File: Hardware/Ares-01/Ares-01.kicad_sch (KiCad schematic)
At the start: 25 parts, among them J1 BTS7960_1, J12 XT60, J13 TCRT5000_1, J14 TCRT5000_2, J15 TCRT5000_3, J2 BTS7960_2, J3 Sharp, J4 Sharp, J5 Sharp, J6 Sharp, J7 Sharp, J8 Qtr8a, J9 Ssd1306 Arduino Pic, SW1 Switch, SW2 SW_Push, SW3 SW_Push, U1 L7805, U3 CD74HC4067M

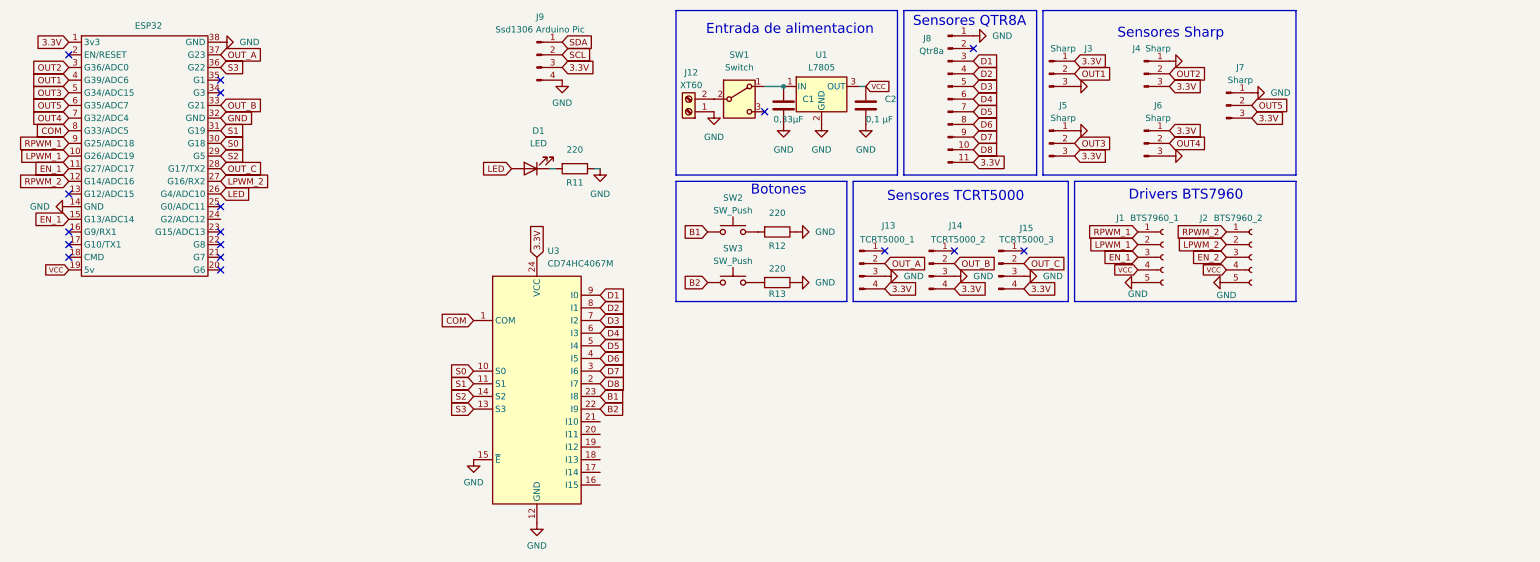
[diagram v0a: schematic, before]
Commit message: primer version del pcb
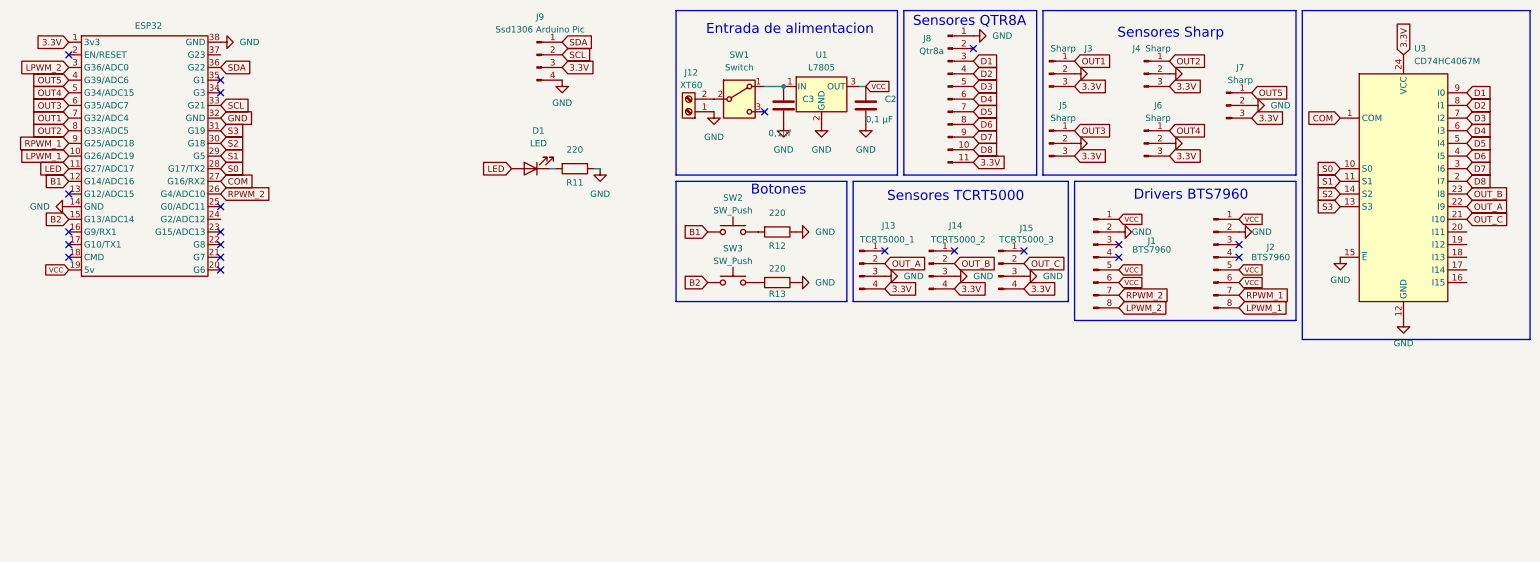
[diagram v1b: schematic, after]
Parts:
- removed C1: 0,33µF, symbol Device:C
- removed J1: BTS7960_1, Connector_IDC:IDC-Header_2x04_P2.54mm_Vertical, symbol Connector:Conn_01x05_Socket
- removed J2: BTS7960_2, Connector_IDC:IDC-Header_2x04_P2.54mm_Vertical, symbol Connector:Conn_01x05_Socket
- added C3: 0,1uf, Capacitor_SMD:C_1206_3216Metric_Pad1.33x1.80mm_HandSolder, symbol Device:C
- added J1, J2: BTS7960, Connector_IDC:IDC-Header_2x04_P2.54mm_Vertical, symbol Connector:Conn_01x08_Pin
- C2: footprint (none) -> Capacitor_SMD:C_1206_3216Metric_Pad1.33x1.80mm_HandSolder
- D1: footprint Connector_JST:JST_EH_S2B-EH_1x02_P2.50mm_Horizontal -> Connector_JST:JST_EH_B2B-EH-A_1x02_P2.50mm_Vertical
- J13, J14, J15: footprint Connector_JST:JST_EH_S4B-EH_1x04_P2.50mm_Horizontal -> Connector_JST:JST_EH_B4B-EH-A_1x04_P2.50mm_Vertical
- J3, J4, J5, J6, J7: footprint Connector_JST:JST_EH_S3B-EH_1x03_P2.50mm_Horizontal -> Connector_JST:JST_EH_B3B-EH-A_1x03_P2.50mm_Vertical
- J8: footprint Connector_JST:JST_EH_S11B-EH_1x11_P2.50mm_Horizontal -> Connector_JST:JST_EH_B10B-EH-A_1x10_P2.50mm_Vertical
- SW1: footprint EESTN5 2:SW_SPDT_TH_Vertical -> EESTN5:SW_SPDT_TH_Vertical
- SW2, SW3: footprint EESTN5 2:PUSH_SWITCH_THT -> EESTN5:PUSH_SWITCH_THT
- U3: footprint Package_SO:SOIC-24W_7.5x15.4mm_P1.27mm -> RamLib:CD74HC4067_module
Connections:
- net 3.3V: now also J3.3 (Pin_3), J6.3 (Pin_3); no longer J3.1 (Pin_1), J6.1 (Pin_1)
- net B1: now also ESP32.12 (G14/ADC16); no longer U3.23 (I8)
- net B2: now also ESP32.15 (G13/ADC14); no longer U3.22 (I9)
- net COM: now also ESP32.27 (G16/RX2); no longer ESP32.8 (G33/ADC5)
- net GND: now also J3.2 (Pin_2), J4.2 (Pin_2), J5.2 (Pin_2), J6.2 (Pin_2), J7.2 (Pin_2), C3.2, J1.2 (Pin_2), J2.2 (Pin_2); no longer J3.3 (Pin_3), J4.1 (Pin_1), J5.1 (Pin_1), J6.3 (Pin_3), J7.1 (Pin_1)
- net LED: now also ESP32.11 (G27/ADC17); no longer ESP32.26 (G4/ADC10)
- net LPWM_1: now also J2.8 (Pin_8)
- net LPWM_2: now also ESP32.3 (G36/ADC0), J1.8 (Pin_8); no longer ESP32.27 (G16/RX2)
- net OUT1: now also ESP32.7 (G32/ADC4), J3.1 (Pin_1); no longer ESP32.4 (G39/ADC6), J3.2 (Pin_2)
- net OUT2: now also ESP32.8 (G33/ADC5), J4.1 (Pin_1); no longer ESP32.3 (G36/ADC0), J4.2 (Pin_2)
- net OUT3: now also ESP32.6 (G35/ADC7), J5.1 (Pin_1); no longer ESP32.5 (G34/ADC15), J5.2 (Pin_2)
- net OUT4: now also ESP32.5 (G34/ADC15), J6.1 (Pin_1); no longer ESP32.7 (G32/ADC4), J6.2 (Pin_2)
- net OUT5: now also ESP32.4 (G39/ADC6), J7.1 (Pin_1); no longer ESP32.6 (G35/ADC7), J7.2 (Pin_2)
- net OUT_A: now also U3.22 (I9); no longer ESP32.37 (G23)
- net OUT_B: now also U3.23 (I8); no longer ESP32.33 (G21)
- net OUT_C: now also U3.21 (I10); no longer ESP32.28 (G17/TX2)
- net RPWM_1: now also J2.7 (Pin_7)
- net RPWM_2: now also ESP32.26 (G4/ADC10), J1.7 (Pin_7); no longer ESP32.12 (G14/ADC16)
- net S0: now also ESP32.28 (G17/TX2); no longer ESP32.30 (G18)
- net S1: now also ESP32.29 (G5); no longer ESP32.31 (G19)
- net S2: now also ESP32.30 (G18); no longer ESP32.29 (G5)
- net S3: now also ESP32.31 (G19); no longer ESP32.36 (G22)
- net SCL: now also ESP32.33 (G21)
- net SDA: now also ESP32.36 (G22)
- net VCC: now also J1.1 (Pin_1), J1.5 (Pin_5), J1.6 (Pin_6), J2.1 (Pin_1), J2.5 (Pin_5), J2.6 (Pin_6)
- net at SW1.1 (A), U1.1 (IN): now also C3.1
- removed net EN_1: ESP32.11 (G27/ADC17), ESP32.15 (G13/ADC14)
- no-connect marks 17 -> 21
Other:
- moved on the sheet: U3

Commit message: primera version del pcb,2
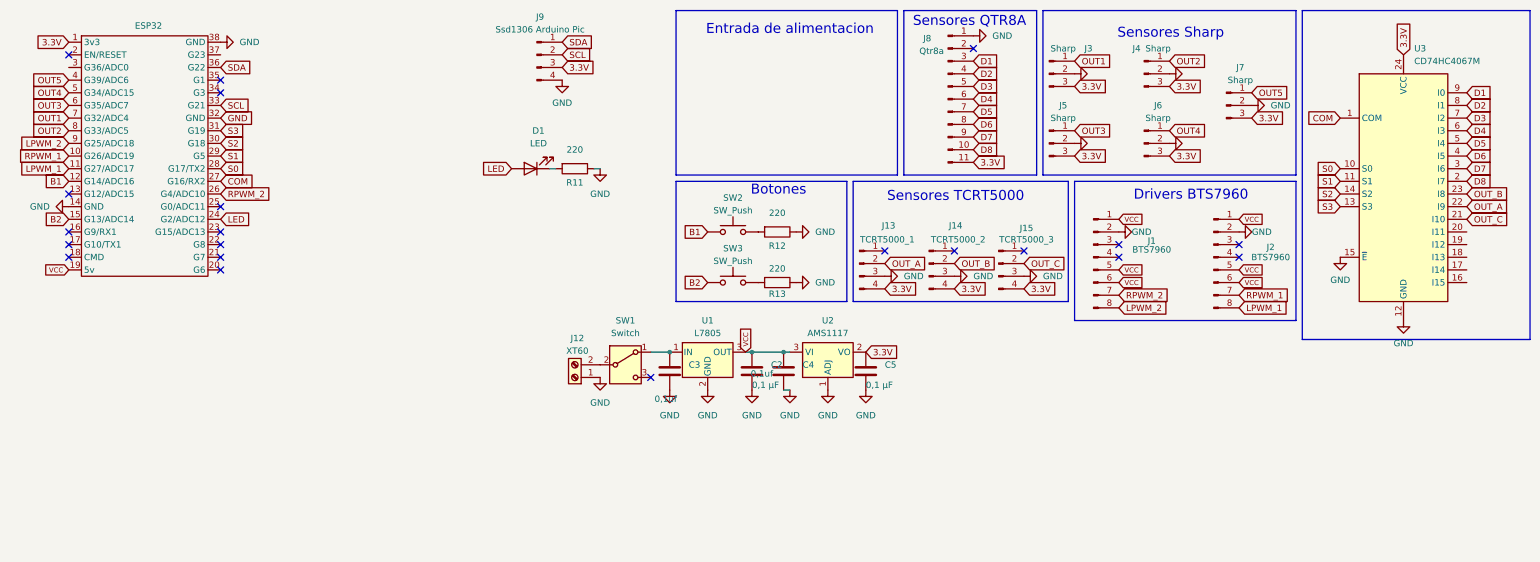
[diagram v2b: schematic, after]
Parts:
- added C4: 0,1uf, Capacitor_SMD:C_1206_3216Metric_Pad1.33x1.80mm_HandSolder, symbol Device:C
- added C5: 0,1 µF, Capacitor_SMD:C_1206_3216Metric_Pad1.33x1.80mm_HandSolder, symbol Device:C
- added U2: AMS1117, Package_TO_SOT_SMD:SOT-223-3_TabPin2, symbol Regulator_Linear:AMS1117
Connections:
- net 3.3V: now also C5.1, U2.2 (VO)
- net GND: now also C4.2, C5.2, U2.1 (ADJ)
- net LED: now also ESP32.24 (G2/ADC12); no longer ESP32.11 (G27/ADC17)
- net LPWM_1: now also ESP32.11 (G27/ADC17); no longer ESP32.10 (G26/ADC19)
- net LPWM_2: now also ESP32.9 (G25/ADC18); no longer ESP32.3 (G36/ADC0)
- net RPWM_1: now also ESP32.10 (G26/ADC19); no longer ESP32.9 (G25/ADC18)
- net VCC: now also C4.1, U2.3 (VI)
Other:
- moved on the sheet: C2, C3, J12, SW1, U1

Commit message: Version 2.1 PCB
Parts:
- J12: footprint Connector_AMASS:AMASS_XT60-F_1x02_P7.20mm_Vertical -> RamLib2:XT30 connector
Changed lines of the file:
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@@
 			)
 		)
-		(property "Footprint" "Connector_AMASS:AMASS_XT60-F_1x02_P7.20mm_Vertical"
+		(property "Footprint" "RamLib2:XT30 connector"
 			(at 127 87.63 0)
 			(effects

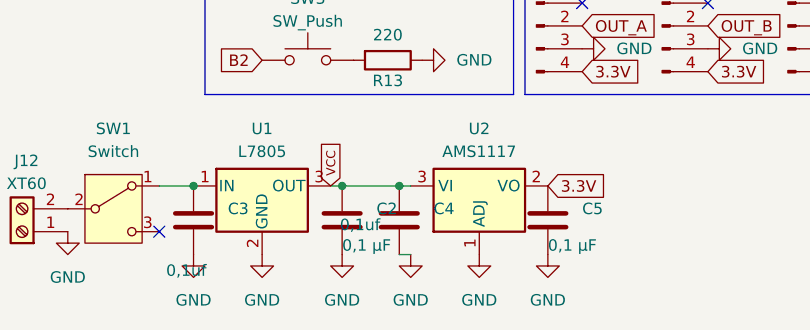
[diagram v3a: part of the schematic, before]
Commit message: version 2.1 PCB
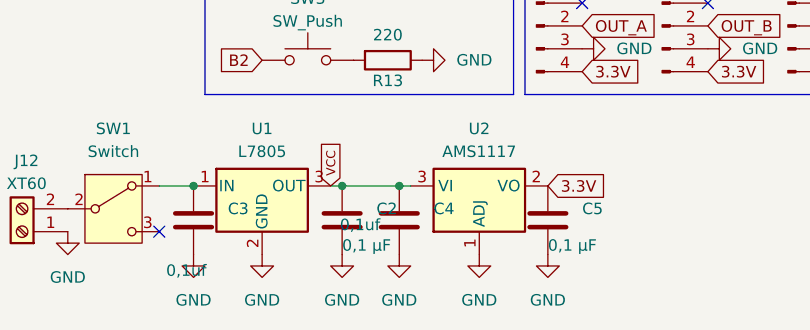
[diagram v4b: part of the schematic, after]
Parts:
- C2, C3, C4, C5: footprint Capacitor_SMD:C_1206_3216Metric_Pad1.33x1.80mm_HandSolder -> Capacitor_SMD:C_0805_2012Metric
- R11, R12, R13: footprint Resistor_SMD:R_1206_3216Metric -> Resistor_SMD:R_0805_2012Metric
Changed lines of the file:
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@@
 		)
 	)
-	(wire
-		(pts
-			(xy 168.91 90.17) (xy 170.18 90.17)
-		)
-		(stroke
-			(width 0)
-			(type default)
-		)
-	)
 	(bus
 		(pts
@@
 			)
 		)
-		(property "Footprint" "Capacitor_SMD:C_1206_3216Metric_Pad1.33x1.80mm_HandSolder"
+		(property "Footprint" "Capacitor_SMD:C_0805_2012Metric"
 			(at 169.8752 90.17 0)
 			(effects
@@
 	(symbol
 		(lib_id "power:GND")
-		(at 170.18 90.17 0)
+		(at 168.91 90.17 0)
 		(unit 1)
 		(exclude_from_sim no)
@@
 		(fields_autoplaced yes)
 		(property "Reference" "#PWR027"
-			(at 170.18 96.52 0)
+			(at 168.91 96.52 0)
 			(effects
 				(font
@@
 		)
 		(property "Value" "GND"
-			(at 170.18 95.25 0)
+			(at 168.91 95.25 0)
 			(effects
 				(font
@@
 		)
 		(property "Footprint" ""
-			(at 170.18 90.17 0)
+			(at 168.91 90.17 0)
 			(effects
 				(font
@@
 		)
 		(property "Datasheet" ""
-			(at 170.18 90.17 0)
+			(at 168.91 90.17 0)
 			(effects
 				(font
@@
 		)
 		(property "Description" "Power symbol creates a global label with name \"GND\" , ground"
-			(at 170.18 90.17 0)
+			(at 168.91 90.17 0)
 			(effects
 				(font
@@
 			)
 		)
-		(property "Footprint" "Capacitor_SMD:C_1206_3216Metric_Pad1.33x1.80mm_HandSolder"
+		(property "Footprint" "Capacitor_SMD:C_0805_2012Metric"
 			(at 186.3852 90.17 0)
 			(effects
@@
 			)
 		)
-		(property "Footprint" "Capacitor_SMD:C_1206_3216Metric_Pad1.33x1.80mm_HandSolder"
+		(property "Footprint" "Capacitor_SMD:C_0805_2012Metric"
 			(at 163.5252 90.17 0)
 			(effects
@@
 			)
 		)
-		(property "Footprint" "Capacitor_SMD:C_1206_3216Metric_Pad1.33x1.80mm_HandSolder"
+		(property "Footprint" "Capacitor_SMD:C_0805_2012Metric"
 			(at 147.0152 90.17 0)
 			(effects
@@
 			)
 		)
-		(property "Footprint" "Resistor_SMD:R_1206_3216Metric"
+		(property "Footprint" "Resistor_SMD:R_0805_2012Metric"
 			(at 167.64 66.802 90)
 			(effects
@@
 			)
 		)
-		(property "Footprint" "Resistor_SMD:R_1206_3216Metric"
+		(property "Footprint" "Resistor_SMD:R_0805_2012Metric"
 			(at 127 43.942 90)
 			(effects
@@
 			)
 		)
-		(property "Footprint" "Resistor_SMD:R_1206_3216Metric"
+		(property "Footprint" "Resistor_SMD:R_0805_2012Metric"
 			(at 167.64 56.642 90)
 			(effects

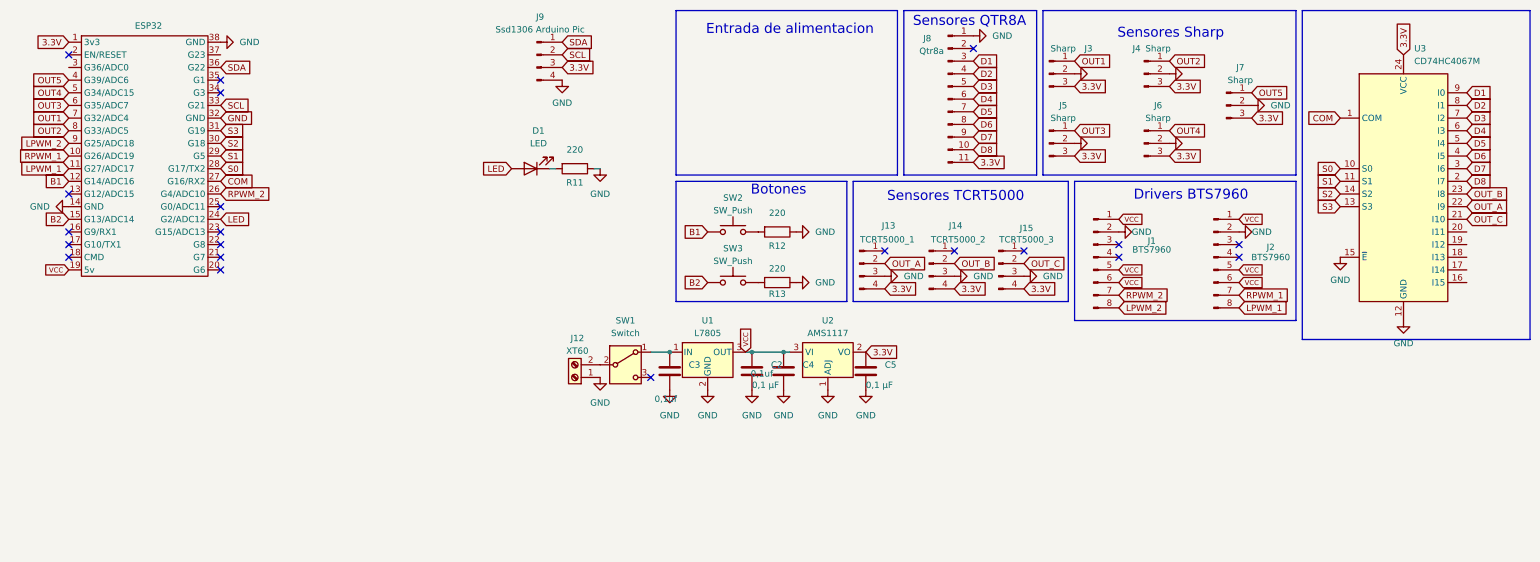
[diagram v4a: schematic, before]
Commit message: version 3 del pcb
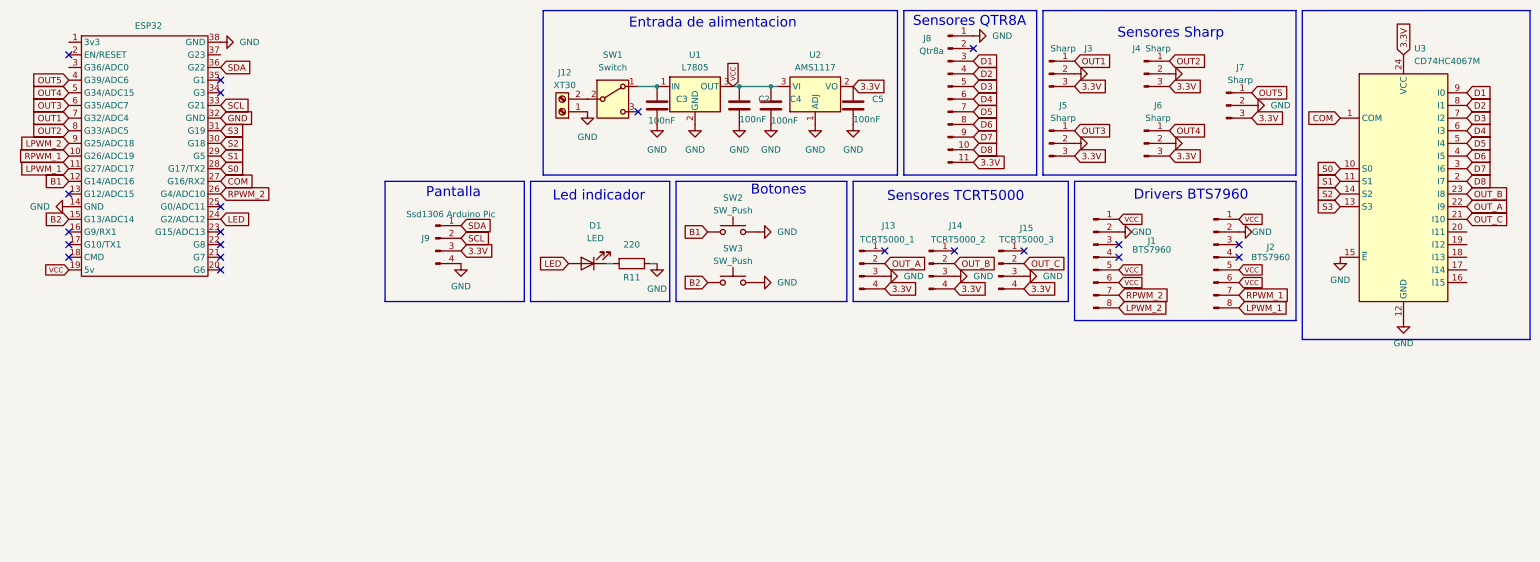
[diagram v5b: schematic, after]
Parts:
- removed R12, R13: 220, Resistor_SMD:R_0805_2012Metric, symbol Device:R
- C2, C5: value 0,1 µF -> 100nF
- C3, C4: value 0,1uf -> 100nF
- J12: value XT60 -> XT30
- J13, J14, J15, J9: footprint Connector_JST:JST_EH_B4B-EH-A_1x04_P2.50mm_Vertical -> Connector_JST:JST_XH_B4B-XH-A_1x04_P2.50mm_Vertical
- J3, J4, J5, J6, J7: footprint Connector_JST:JST_EH_B3B-EH-A_1x03_P2.50mm_Vertical -> Connector_JST:JST_XH_B3B-XH-A_1x03_P2.50mm_Vertical
- J8: footprint Connector_JST:JST_EH_B10B-EH-A_1x10_P2.50mm_Vertical -> Connector_JST:JST_XH_B10B-XH-A_1x10_P2.50mm_Vertical
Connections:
- net 3.3V: no longer ESP32.1 (3v3)
- net GND: now also SW2.2, SW3.2
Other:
- note added: "Led indicador"
- note added: "Pantalla"
- moved on the sheet: C2, C3, C4, C5, D1, J12, J9, R11, SW1, U1, U2

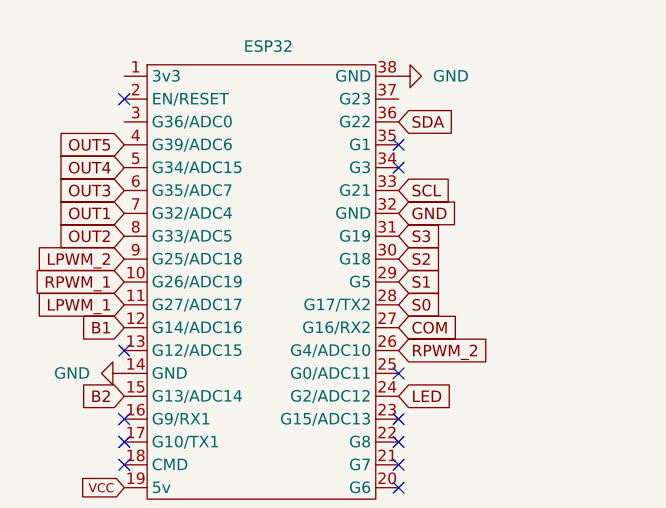
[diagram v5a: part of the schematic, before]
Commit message: Se subio las cosas faltantes
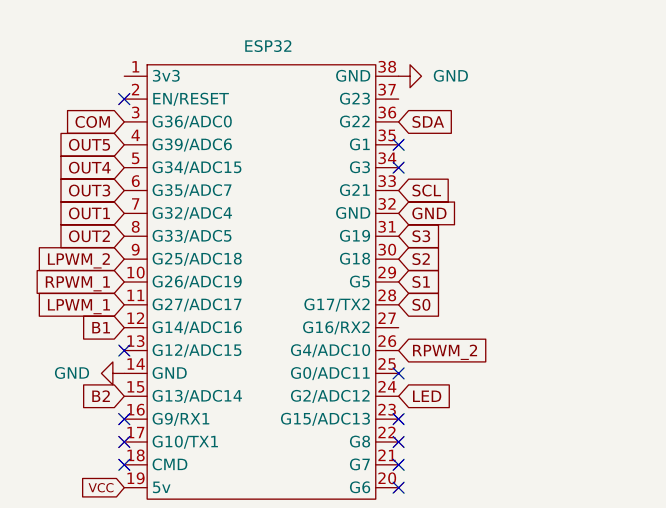
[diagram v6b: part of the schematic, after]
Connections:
- net COM: now also ESP32.3 (G36/ADC0); no longer ESP32.27 (G16/RX2)
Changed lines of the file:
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@@
 	(global_label "COM"
 		(shape input)
-		(at 55.88 48.26 0)
+		(at 25.4 25.4 180)
 		(fields_autoplaced yes)
 		(effects
@@
 				(size 1.27 1.27)
 			)
-			(justify left)
+			(justify right)
 		)
 		(property "Intersheetrefs" "${INTERSHEET_REFS}"
-			(at 62.9171 48.26 0)
+			(at 18.3629 25.4 0)
 			(effects
 				(font
 					(size 1.27 1.27)
 				)
-				(justify left)
+				(justify right)
 				(hide yes)
 			)
